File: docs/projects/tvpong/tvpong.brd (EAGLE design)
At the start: 50.5 x 61 mm, 19 parts, among them Q1 12MHz, X3 AUDIO, X4 VIDEO

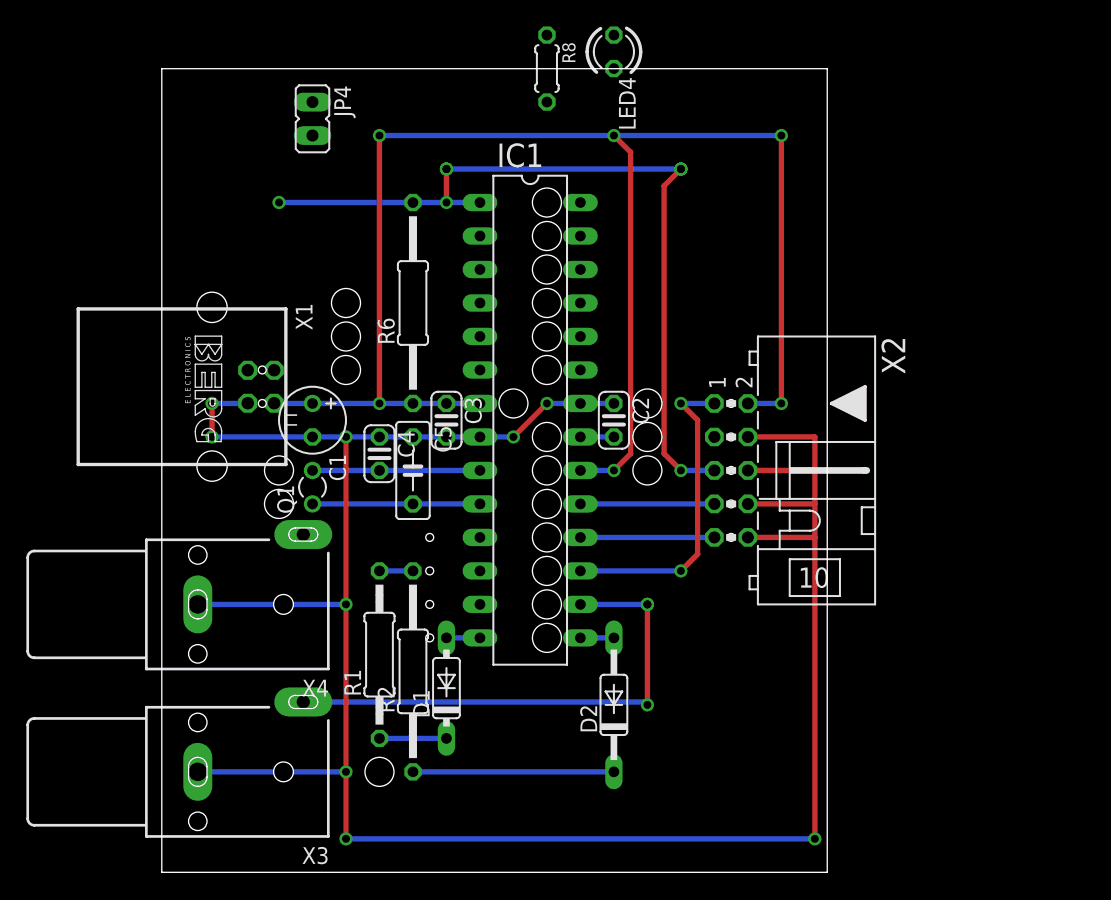
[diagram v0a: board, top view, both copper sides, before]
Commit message: pong
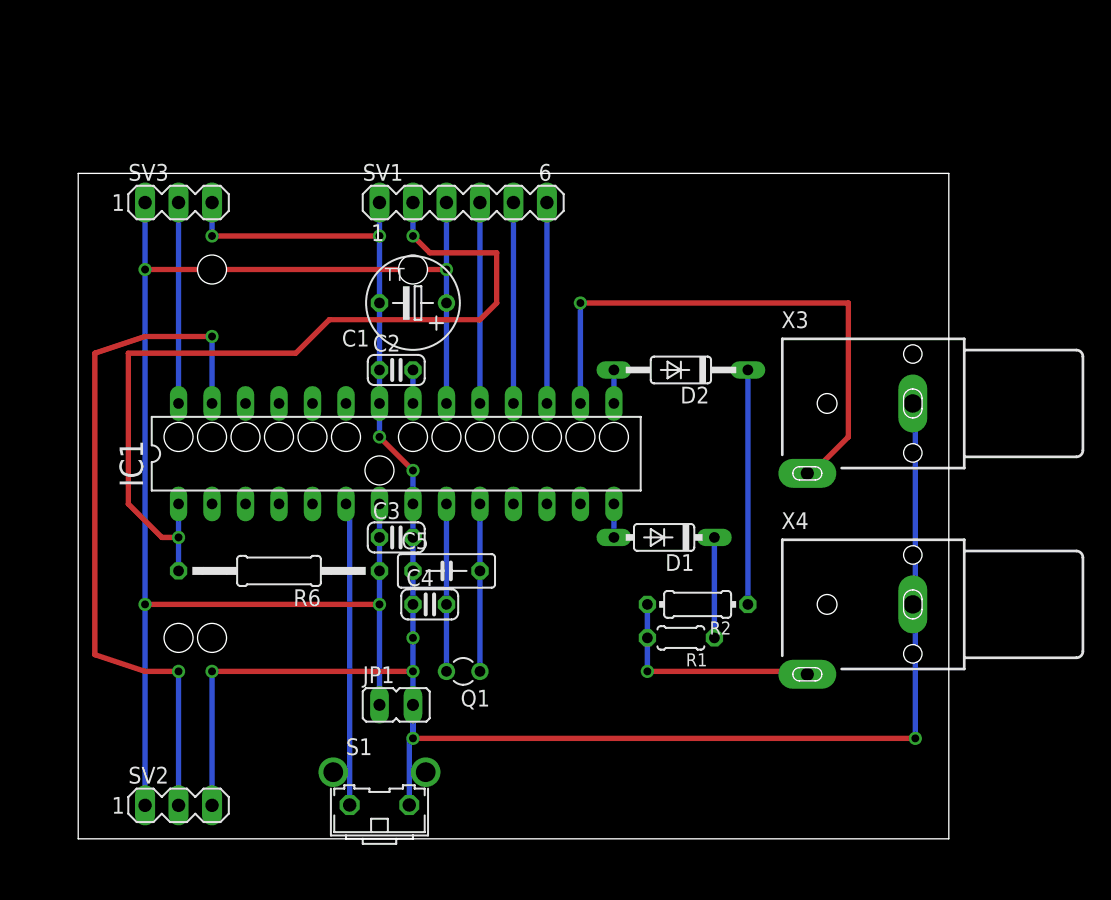
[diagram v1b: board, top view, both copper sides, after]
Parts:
- removed JP4: Reset, jumper:JP1
- removed LED4: POW USB, led:LED3MM
- removed R8: 1k, rcl:0204/5
- removed X1: (no value), con-berg:PN61729
- removed X2: (no value), con-harting-ml:ML10L
- added JP1: (no value), jumper:JP1
- added S1: (no value), switch-omron:B3F-31XX
- added SV1: ISP, con-lstb:MA06-1
- added SV2: POT1, con-lstb:MA03-1
- added SV3: POT2, con-lstb:MA03-1
- C1: device rcl:TT2D5 -> rcl:TT5D7
- Q1: value 12MHz -> 20MHz
- R1: device rcl:0207/12 -> rcl:0204/5
- R2: device rcl:0207/15 -> rcl:0204/7
- moved X3 68.2 mm to (69.8, 35.6), turned to 270 degrees
- moved X4 62.2 mm to (69.8, 20.3), turned to 270 degrees
- moved D2 25.9 mm to (48.3, 38.1), turned to 180 degrees
- moved R1 22.9 mm to (48.3, 17.8), turned to 180 degrees
- moved R6 22.7 mm to (17.8, 22.9), turned to 180 degrees
- moved R2 22.2 mm to (49.5, 20.3), turned to 180 degrees
- moved D1 20.1 mm to (47.0, 25.4), turned to 180 degrees
- moved Q1 18.1 mm to (31.8, 15.2), turned to 180 degrees
- moved C2 16.9 mm to (26.7, 38.1), turned to 0 degrees
- moved C4 12.0 mm to (29.2, 20.3), turned to 0 degrees
- moved C1 11.7 mm to (27.9, 43.2), turned to 180 degrees
- moved IC1 10.5 mm to (26.7, 31.8), turned to 0 degrees
- moved C3 9.67 mm to (26.7, 25.4), turned to 0 degrees
- moved C5 8.03 mm to (30.5, 22.9), turned to 0 degrees
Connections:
- removed net UNUSED: X2.3
- new net N$3: IC1.27, SV2.2
- new net N$9: IC1.6, S1.1
- net +5V: now also JP1.1, SV1.3, SV2.1, SV3.1; no longer R8.1, X1.1, X2.2
- net GND: now also JP1.2, S1.2, SV1.1, SV2.3, SV3.3; no longer JP4.2, LED4.K, X1.4, X2.10, X2.4, X2.6, X2.8
- net MISO: now also SV1.5; no longer X2.9
- net MOSI: now also SV1.6; no longer X2.1
- net N$4: now also IC1.28, SV3.2; no longer LED4.A, R8.2
- net RST: now also SV1.2; no longer JP4.1, X2.5
- net SCK: now also SV1.4; no longer X2.7
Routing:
- net N$3: track 0.00 -> 53.8 mm, vias 0 -> 2
- net N$9: track 0.00 -> 23.1 mm, vias 1 -> 0
- net GND: track 176.1 -> 153.7 mm
- net N$4: track 0.00 -> 15.2 mm
- net N$11: track 2.54 -> 17.4 mm, vias 0 -> 1
- net MOSI: track 23.9 -> 15.2 mm, vias 2 -> 0
- net SCK: track 10.2 -> 15.2 mm
- net MISO: track 10.2 -> 15.2 mm
- net N$15: track 39.0 -> 41.7 mm, vias 2 -> 1
- net N$7: track 15.2 -> 17.8 mm
- net N$6: track 5.08 -> 7.62 mm
- net RST: track 62.0 -> 64.1 mm, vias 5 -> 2
- net +5V: track 118.3 -> 116.8 mm, vias 6 -> 4
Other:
- board size 50.5 x 61 mm -> 66 x 50.5 mm
